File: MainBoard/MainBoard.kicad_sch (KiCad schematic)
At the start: 19 parts, among them J1 1761681-3, U1 TL072CP

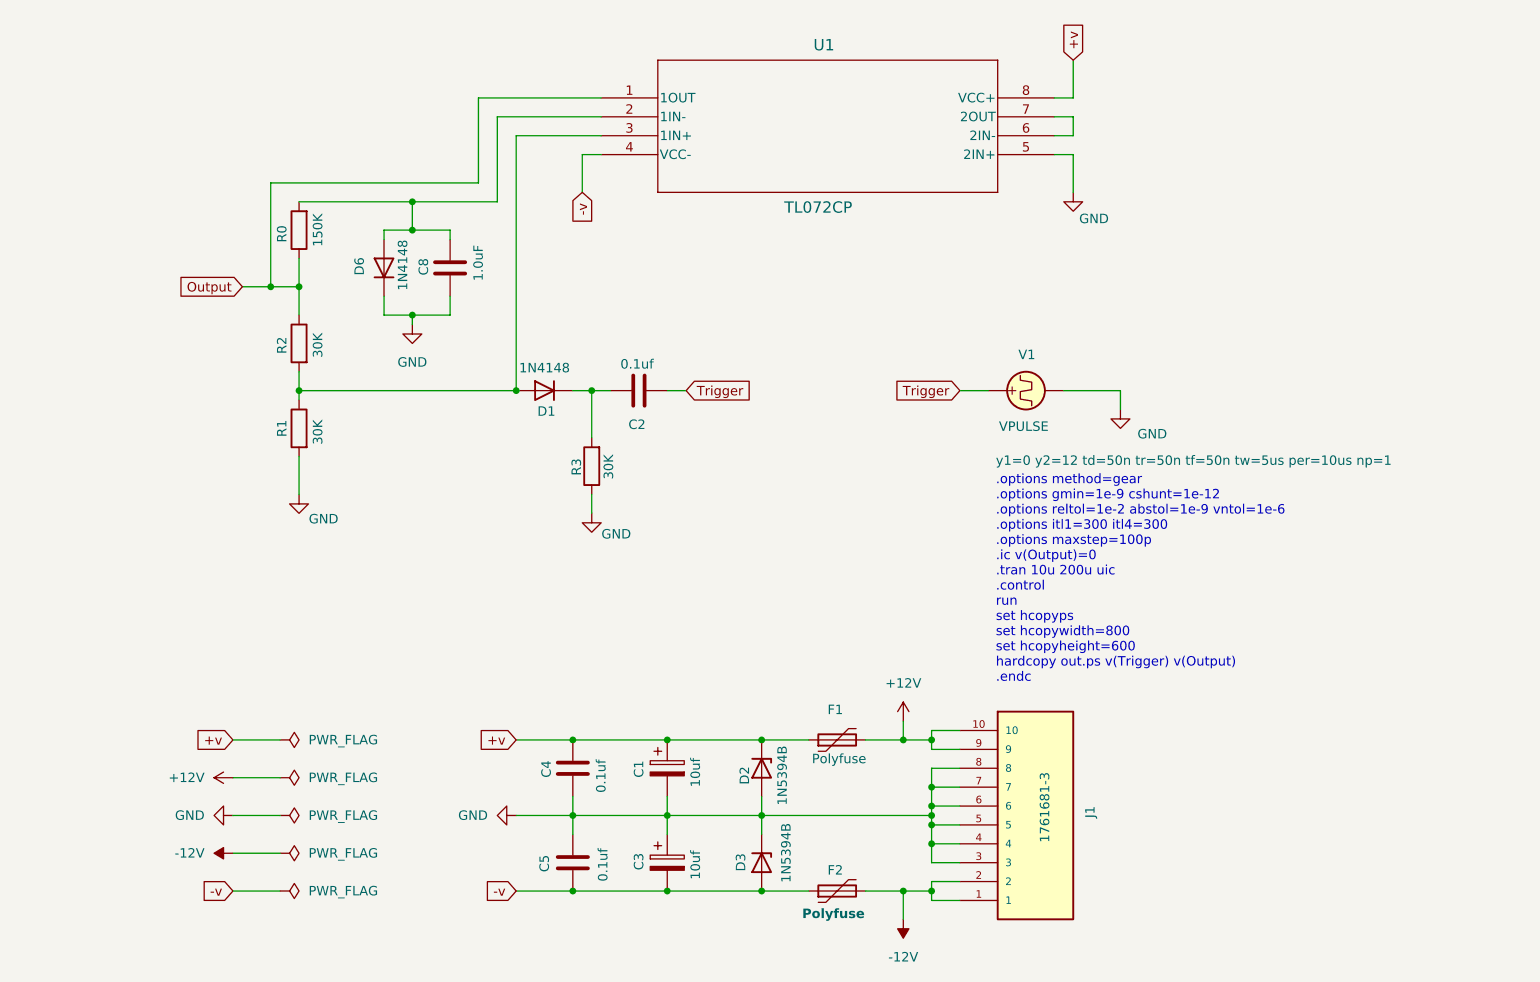
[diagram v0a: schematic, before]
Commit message: some updates for clarity
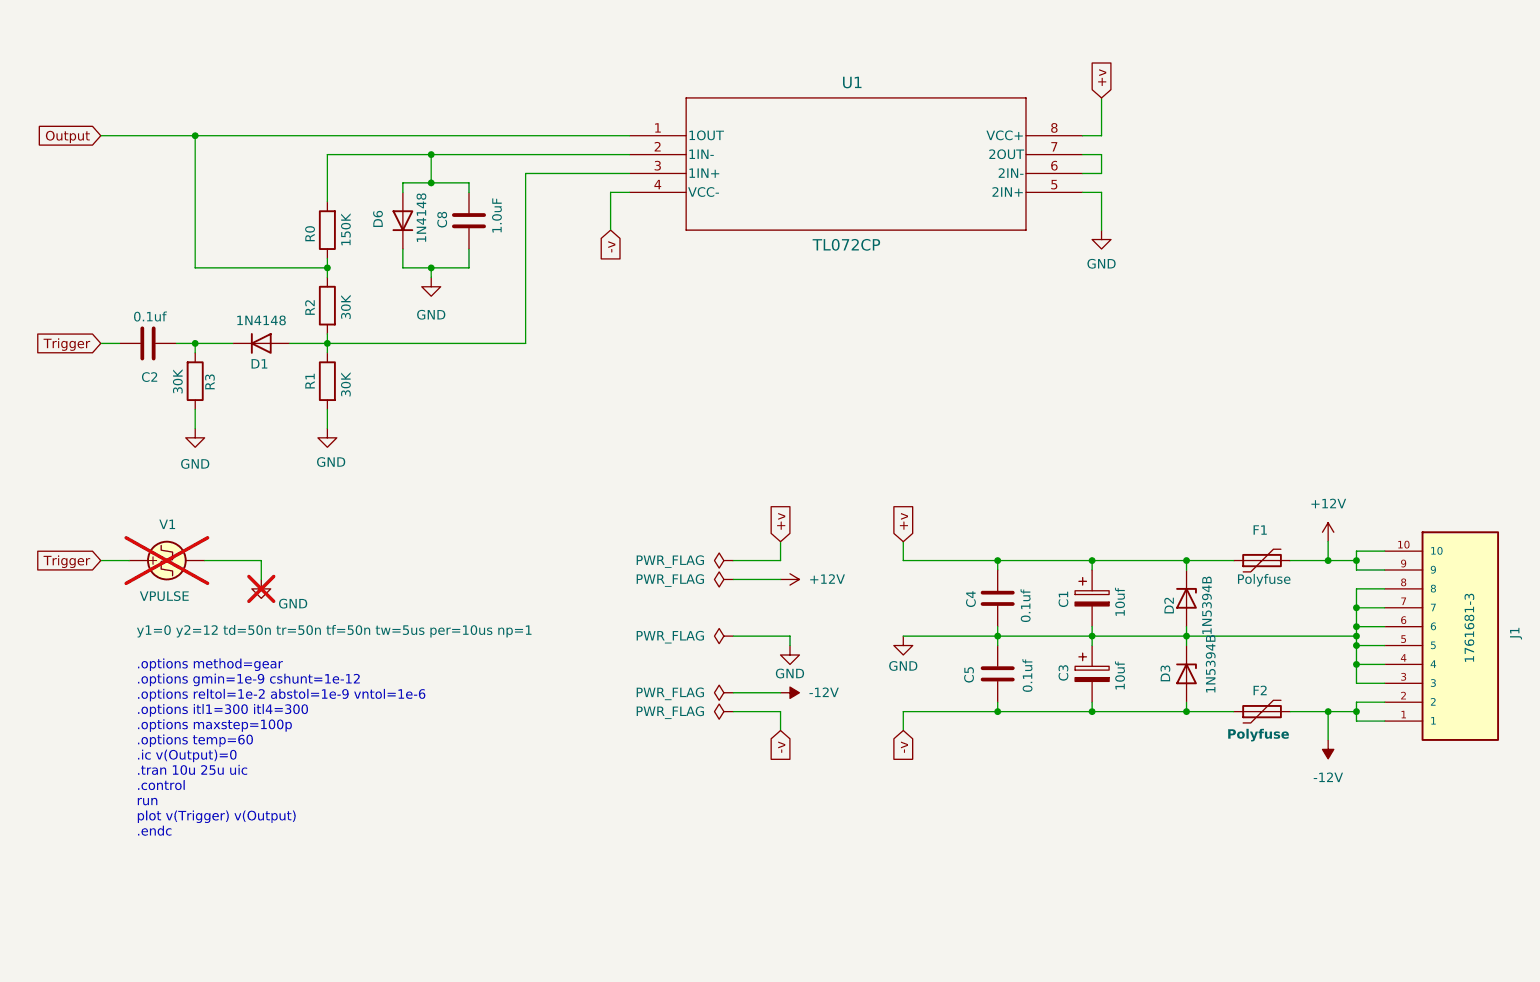
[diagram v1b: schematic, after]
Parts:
- V1: now not fitted; now left out of the parts list
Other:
- note added: ".options method=gear .options gmin=1e-9 cshunt=1e-12 .options reltol=1e-2 abstol=1e-9 vntol=1e-6 .options itl1=300 itl4=300 .options maxstep=100p .options temp=60 .ic v(Output)=0 .tran 10u 25u uic .control run plot v(Trigger) v(Output) .endc"
- note removed: ".options method=gear .options gmin=1e-9 cshunt=1e-12 .options reltol=1e-2 abstol=1e-9 vntol=1e-6 .options itl1=300 itl4=300 .options maxstep=100p .ic v(Output)=0 .tran 10u 200u uic .control run set hcopyps set hcopywidth=800 set hcopyheight=600 hardcopy out.ps v(Trigger) v(Output) .endc"
- moved on the sheet: C1, C2, C3, C4, C5, C8, D1, D2, D3, D6, F1, F2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
